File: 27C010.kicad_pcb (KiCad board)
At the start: 2 copper layers, 21.3 x 41.1 mm, 3 parts, among them J1 Conn_01x16_Male, J2 Conn_01x16_Male, U1 TC571001

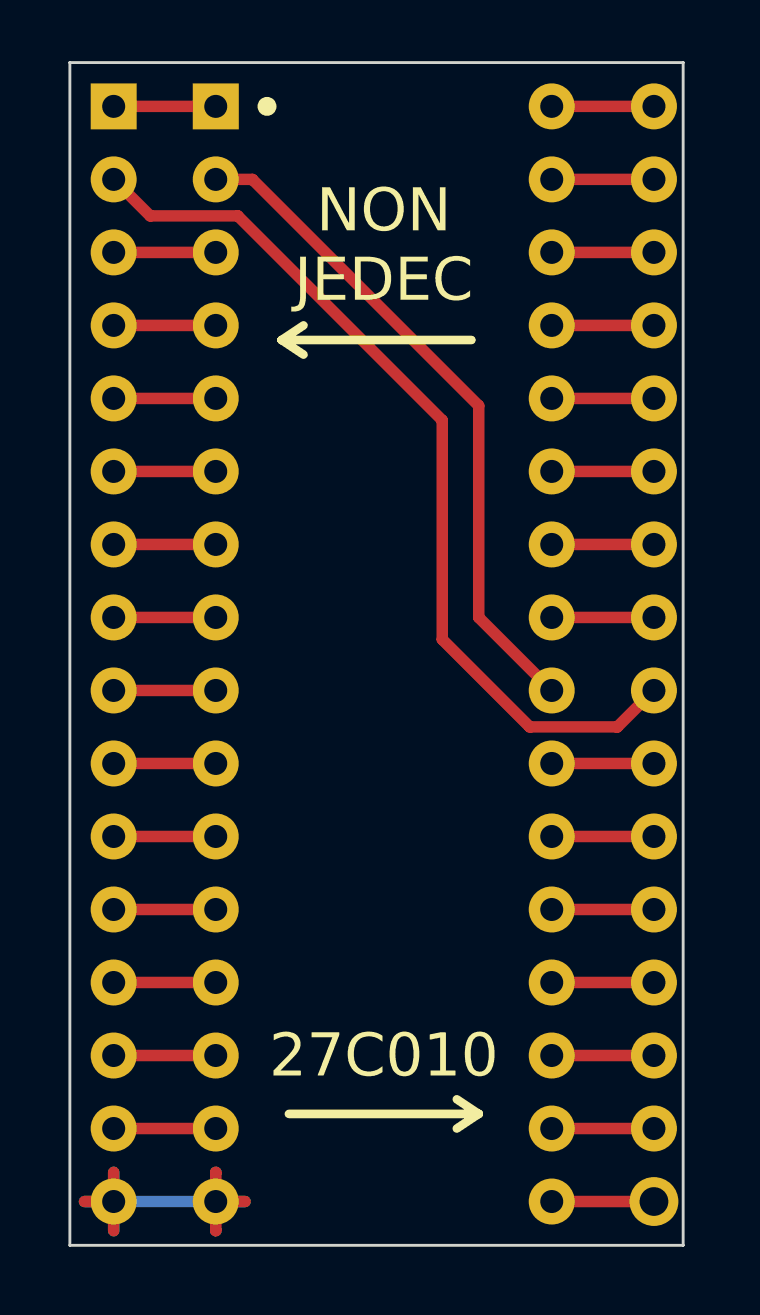
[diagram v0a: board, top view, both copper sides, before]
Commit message: done
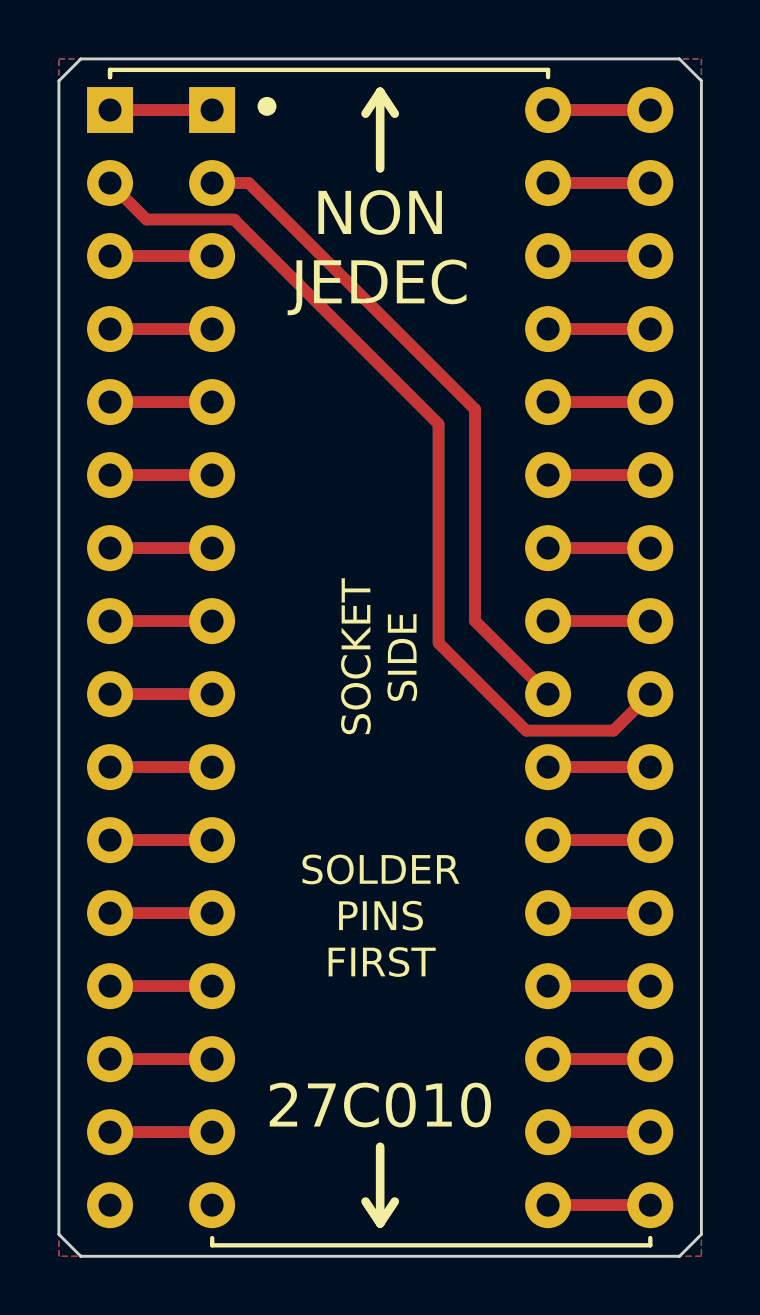
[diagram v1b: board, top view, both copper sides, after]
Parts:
- moved U1 0.18 mm to (98.4, 64.9)
- moved J1 0.18 mm to (102.0, 64.9)
- moved J2 0.18 mm to (117.2, 103.0)
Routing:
- net /~{OE}: track 31.7 -> 63.3 mm
- net /A16: track 23.4 -> 46.7 mm
- net /GND: track 15.8 -> 0.00 mm
- net /VPP: track 3.55 -> 7.10 mm
- net /D2: track 3.55 -> 7.10 mm
- net /D1: track 3.55 -> 7.10 mm
- net /D0: track 3.55 -> 7.10 mm
- net /A7: track 3.55 -> 7.10 mm
- net /A6: track 3.55 -> 7.10 mm
- net /A5: track 3.55 -> 7.10 mm
- net /A4: track 3.55 -> 7.10 mm
- net /A3: track 3.55 -> 7.10 mm
- net /A2: track 3.55 -> 7.10 mm
- net /A15: track 3.55 -> 7.10 mm
- net /A12: track 3.55 -> 7.10 mm
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- added copper zone on B.Cu, net /GND
- added copper zone on F.Cu, net /GND
- removed copper zone on B.Cu, net (none)
- removed copper zone on F.Cu, net (none)
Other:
- board size 21.3 x 41.1 mm -> 22.4 x 41.7 mm
- board text added: "PIN SIDE"
- board text added: "SOCKET SIDE"
- board text added: "SOLDER PINS FIRST"
